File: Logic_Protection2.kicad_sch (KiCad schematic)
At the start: 16 parts

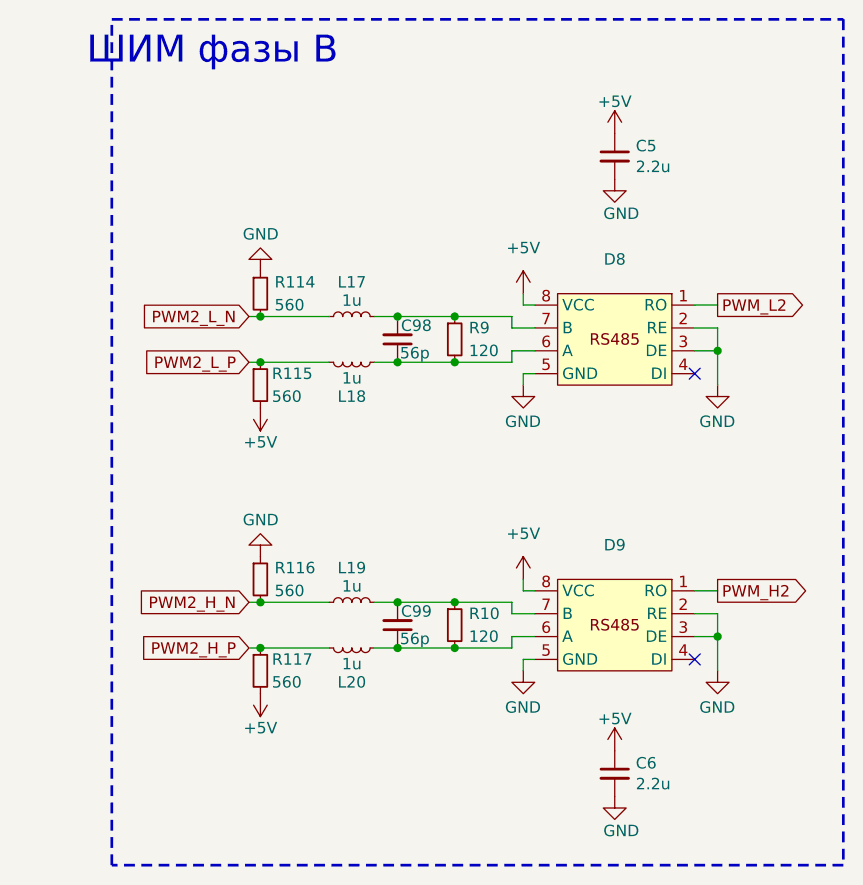
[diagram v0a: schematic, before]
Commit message: VER2.2.1: создал папку для производственных доков
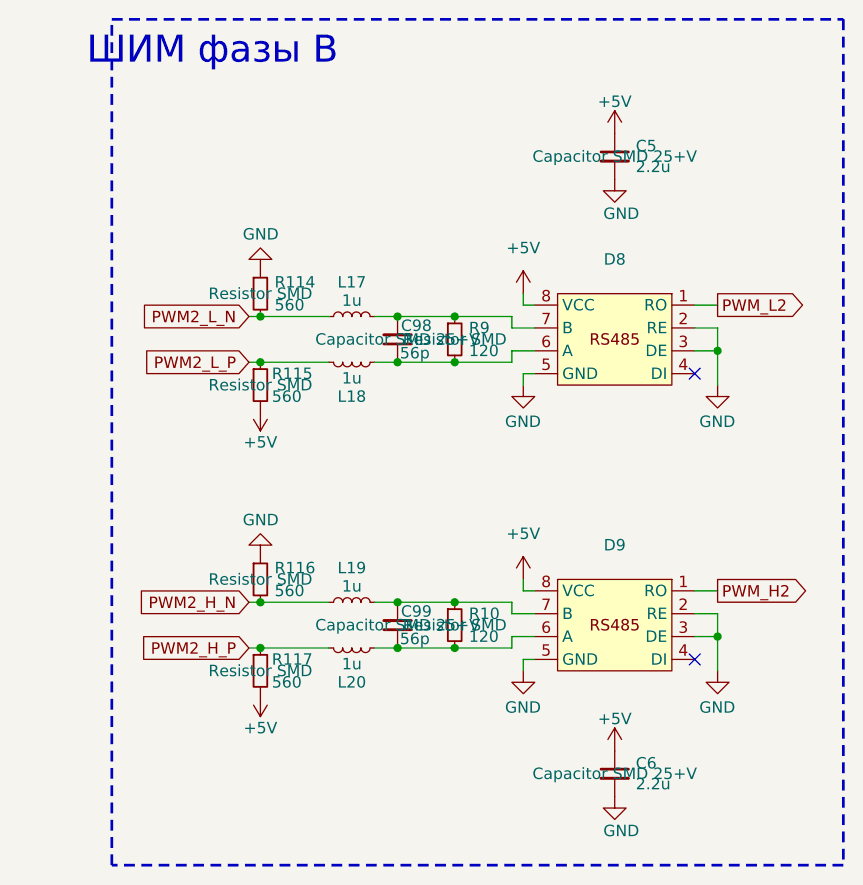
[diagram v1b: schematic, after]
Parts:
- C5, C6, C98, C99: Description P/N (none) -> Capacitor SMD 25+V
- R10, R114, R115, R116, R117, R9: Description P/N (none) -> Resistor SMD
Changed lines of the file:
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@@
 			)
 		)
-		(property "Description P/N" ""
+		(property "Description P/N" "Capacitor SMD 25+V"
 			(at 140.97 86.36 0)
 			(effects
@@
 			)
 		)
-		(property "Description P/N" ""
+		(property "Description P/N" "Capacitor SMD 25+V"
 			(at 140.97 118.11 0)
 			(effects
@@
 			)
 		)
-		(property "Description P/N" ""
+		(property "Description P/N" "Resistor SMD"
 			(at 125.73 123.19 0)
 			(effects
@@
 			)
 		)
-		(property "Description P/N" ""
+		(property "Description P/N" "Resistor SMD"
 			(at 147.32 86.36 0)
 			(effects
@@
 			)
 		)
-		(property "Description P/N" ""
+		(property "Description P/N" "Capacitor SMD 25+V"
 			(at 165.1 134.62 0)
 			(effects
@@
 			)
 		)
-		(property "Description P/N" ""
+		(property "Description P/N" "Resistor SMD"
 			(at 125.73 91.44 0)
 			(effects
@@
 			)
 		)
-		(property "Description P/N" ""
+		(property "Description P/N" "Resistor SMD"
 			(at 125.73 81.28 0)
 			(effects
@@
 			)
 		)
-		(property "Description P/N" ""
+		(property "Description P/N" "Capacitor SMD 25+V"
 			(at 165.1 66.04 0)
 			(effects
@@
 			)
 		)
-		(property "Description P/N" ""
+		(property "Description P/N" "Resistor SMD"
 			(at 125.73 113.03 0)
 			(effects
@@
 			)
 		)
-		(property "Description P/N" ""
+		(property "Description P/N" "Resistor SMD"
 			(at 147.32 118.11 0)
 			(effects
